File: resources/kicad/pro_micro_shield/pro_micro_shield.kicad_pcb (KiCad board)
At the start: 2 copper layers, 34.5 x 45.8 mm, 8 parts, among them J1 Conn_01x06_Female, J2 Conn_01x12_Female, J3 Conn_01x09_Female, U1 ProMicro

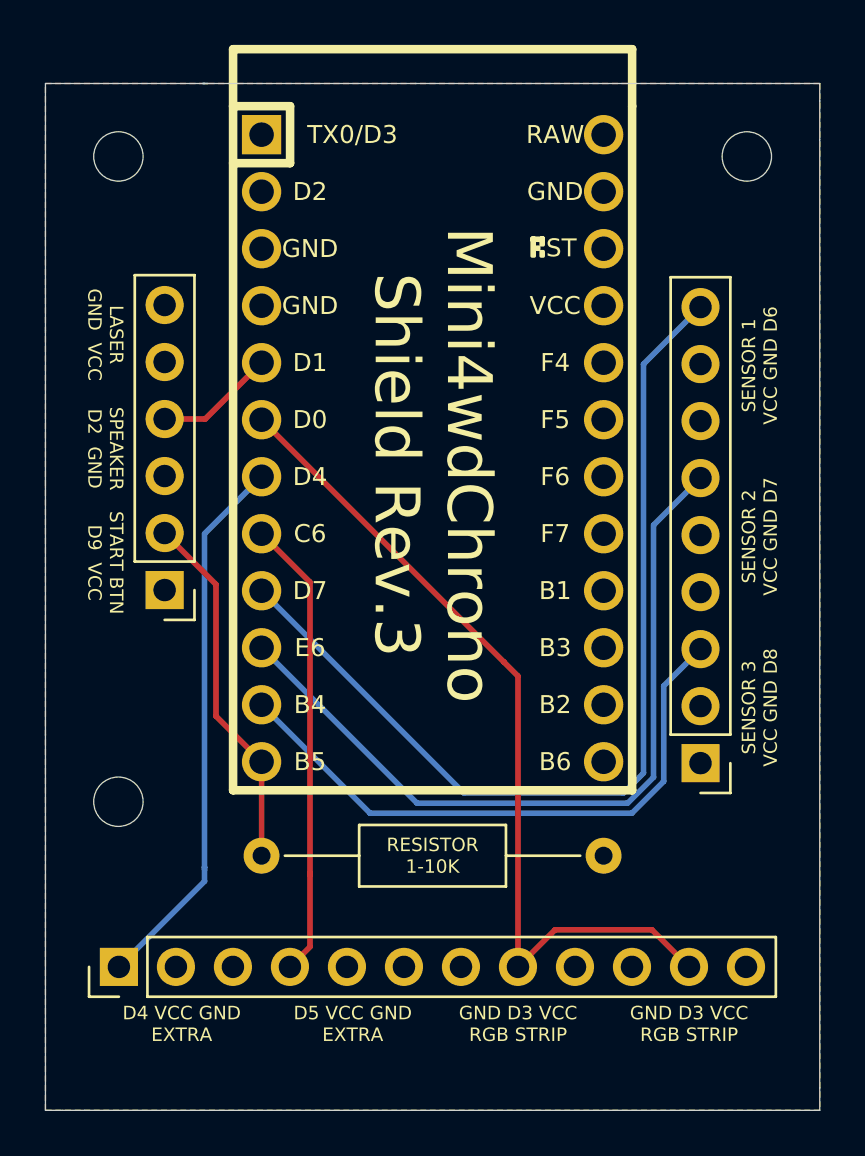
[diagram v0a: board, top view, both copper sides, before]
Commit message: shield revision 3
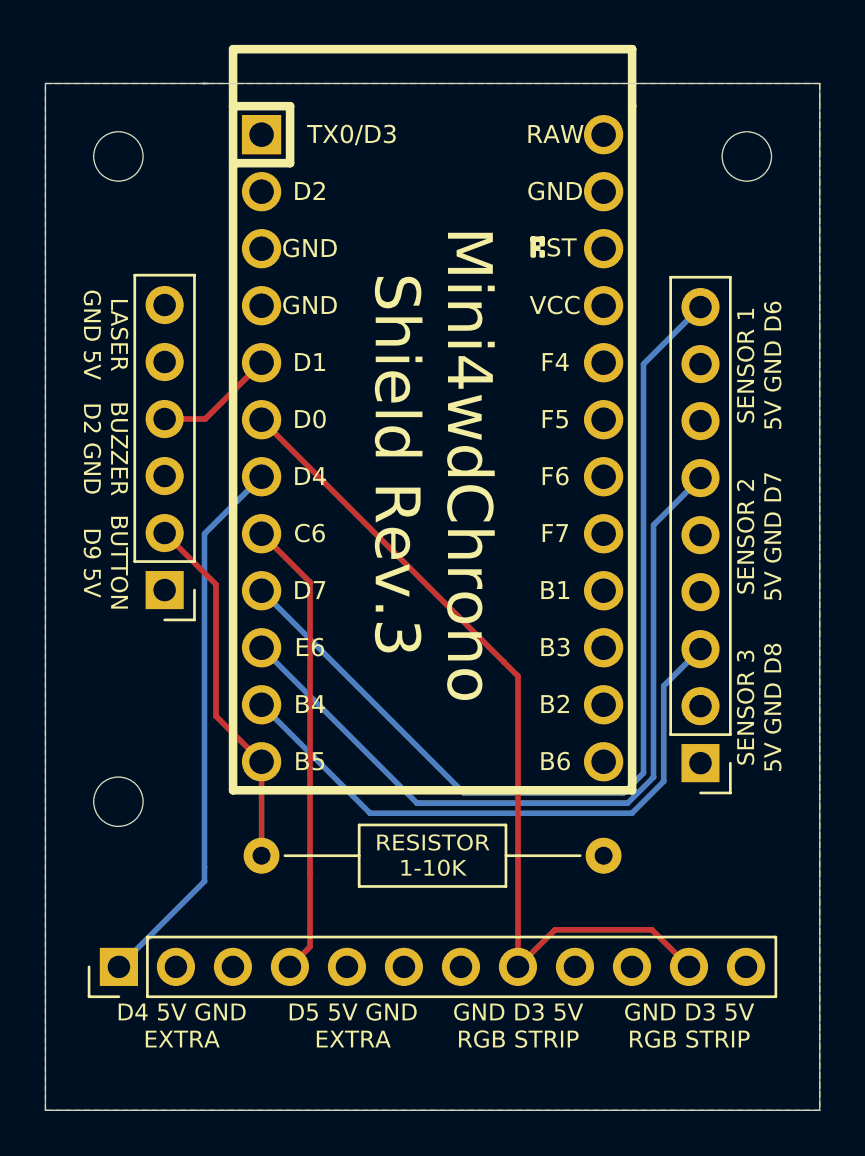
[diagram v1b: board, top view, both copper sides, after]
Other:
- board text added: "BUTTON D9 5V"
- board text added: "BUZZER D2 GND"
- board text added: "D4 5V GND EXTRA"
- board text added: "D5 5V GND EXTRA"
- board text added: "GND D3 5V RGB STRIP"
- board text added: "LASER GND 5V"
- board text added: "SENSOR 1 5V GND D6"
- board text added: "SENSOR 2 5V GND D7"
- board text added: "SENSOR 3 5V GND D8"
- board text removed: "D4 VCC GND EXTRA"
- board text removed: "D5 VCC GND EXTRA"
- board text removed: "GND D3 VCC RGB STRIP"
- board text removed: "LASER GND VCC"
- board text removed: "SENSOR 1 VCC GND D6"
- board text removed: "SENSOR 2 VCC GND D7"
- board text removed: "SENSOR 3 VCC GND D8"
- board text removed: "SPEAKER D2 GND"
- board text removed: "START BTN D9 VCC"
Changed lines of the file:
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@@
     (effects (font (size 0.6 0.6) (thickness 0.15)) (justify mirror))
   )
-  (gr_text "LASER\nGND  VCC" (at 159.9184 81.9404 270) (layer "F.SilkS")
-    (effects (font (size 0.6 0.6) (thickness 0.15)))
+  (gr_text "LASER\nGND 5V" (at 159.9184 81.9404 270) (layer "F.SilkS")
+    (effects (font (size 0.75 0.75) (thickness 0.15)))
   )
-  (gr_text "SENSOR 3\nVCC GND D8" (at 189.0776 98.552 90) (layer "F.SilkS")
-    (effects (font (size 0.6 0.6) (thickness 0.15)))
+  (gr_text "SENSOR 3\n5V GND D8" (at 189.0776 98.552 90) (layer "F.SilkS")
+    (effects (font (size 0.75 0.75) (thickness 0.15)))
   )
-  (gr_text "GND D3 VCC\nRGB STRIP" (at 185.928 112.649) (layer "F.SilkS")
-    (effects (font (size 0.6 0.6) (thickness 0.15)))
+  (gr_text "GND D3 5V\nRGB STRIP" (at 185.928 112.75) (layer "F.SilkS")
+    (effects (font (size 0.75 0.75) (thickness 0.15)))
   )
-  (gr_text "GND D3 VCC\nRGB STRIP" (at 178.308 112.649) (layer "F.SilkS")
-    (effects (font (size 0.6 0.6) (thickness 0.15)))
+  (gr_text "GND D3 5V\nRGB STRIP" (at 178.308 112.75) (layer "F.SilkS")
+    (effects (font (size 0.75 0.75) (thickness 0.15)))
   )
-  (gr_text "SENSOR 2\nVCC GND D7" (at 189.0776 90.932 90) (layer "F.SilkS")
-    (effects (font (size 0.6 0.6) (thickness 0.15)))
+  (gr_text "SENSOR 2\n5V GND D7" (at 189.0776 90.932 90) (layer "F.SilkS")
+    (effects (font (size 0.75 0.75) (thickness 0.15)))
   )
   (gr_text "Mini4wdChrono\nShield Rev.3" (at 174.5 87.75 270) (layer "F.SilkS")
@@
   )
   (gr_text "RESISTOR\n1-10K" (at 174.498 105.156) (layer "F.SilkS")
-    (effects (font (size 0.6 0.6) (thickness 0.15)))
+    (effects (font (size 0.7 0.75) (thickness 0.15)))
   )
-  (gr_text "D5 VCC GND\nEXTRA" (at 170.942 112.649) (layer "F.SilkS")
-    (effects (font (size 0.6 0.6) (thickness 0.15)))
+  (gr_text "D5 5V GND\nEXTRA" (at 170.942 112.75) (layer "F.SilkS")
+    (effects (font (size 0.75 0.75) (thickness 0.15)))
   )
-  (gr_text "D4 VCC GND\nEXTRA" (at 163.322 112.649) (layer "F.SilkS")
-    (effects (font (size 0.6 0.6) (thickness 0.15)))
+  (gr_text "D4 5V GND\nEXTRA" (at 163.322 112.75) (layer "F.SilkS")
+    (effects (font (size 0.75 0.75) (thickness 0.15)))
   )
-  (gr_text "START BTN\nD9  VCC" (at 159.9184 92.1004 -90) (layer "F.SilkS")
-    (effects (font (size 0.6 0.6) (thickness 0.15)))
+  (gr_text "BUTTON\nD9 5V" (at 159.9184 92.1004 -90) (layer "F.SilkS")
+    (effects (font (size 0.75 0.75) (thickness 0.15)))
   )
-  (gr_text "SENSOR 1\nVCC GND D6" (at 189.0776 83.312 90) (layer "F.SilkS")
-    (effects (font (size 0.6 0.6) (thickness 0.15)))
+  (gr_text "SENSOR 1\n5V GND D6" (at 189.0776 83.312 90) (layer "F.SilkS")
+    (effects (font (size 0.75 0.75) (thickness 0.15)))
   )
-  (gr_text "SPEAKER\nD2  GND" (at 159.9184 87.0204 270) (layer "F.SilkS")
-    (effects (font (size 0.6 0.6) (thickness 0.15)))
+  (gr_text "BUZZER\nD2 GND" (at 159.9184 87.0204 270) (layer "F.SilkS")
+    (effects (font (size 0.75 0.75) (thickness 0.15)))
   )
   (segment (start 166.88 100.97) (end 166.88 105.154) (width 0.25) (layer "F.Cu") (net 3))
@@
   (segment (start 179.954 108.458) (end 184.272 108.458) (width 0.25) (layer "F.Cu") (net 5))
   (segment (start 168.143 110.109) (end 169.037 109.215) (width 0.25) (layer "F.Cu") (net 6))
-  (segment (start 169.037 106.045) (end 169.037 105.918) (width 0.25) (layer "F.Cu") (net 6))
   (segment (start 169.037 92.967) (end 166.88 90.81) (width 0.25) (layer "F.Cu") (net 6))
   (segment (start 169.037 109.215) (end 169.037 105.918) (width 0.25) (layer "F.Cu") (net 6))
@@
   (segment (start 164.338 90.812) (end 166.88 88.27) (width 0.25) (layer "B.Cu") (net 7))
   (segment (start 164.338 106.299) (end 164.338 105.664) (width 0.25) (layer "B.Cu") (net 7))
-  (segment (start 164.338 105.791) (end 164.338 105.664) (width 0.25) (layer "B.Cu") (net 7))
   (segment (start 184.796 101.844396) (end 183.378396 103.262) (width 0.25) (layer "B.Cu") (net 8))
   (segment (start 183.378396 103.262) (end 171.712 103.262) (width 0.25) (layer "B.Cu") (net 8))
